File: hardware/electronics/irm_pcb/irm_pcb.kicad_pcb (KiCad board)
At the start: 2 copper layers, 63 parts, among them IC1 23LC1024, J1 Conn_01x04, J10 Conn_02x05_Counter_Clockwise, J11 Conn_01x04, J12 Conn_01x06, J13 Conn_01x06, J14 Conn_01x10, J16 Screw_Terminal_01x02, J17 Conn_01x06, J2 JUMPER_OPEN, J3 JUMPER_CLOSED, J4 JUMPER_CLOSED, J5 AudioJack3_Switch, J6 Screw_Terminal_1x02, J7 Screw_Terminal_1x02, J8 Conn_01x04, J9 Conn_02x15_Top_Bottom, SW1 RST, SW2 0, U1 LM1117-1.8, U2 VS1053B, U3 74LS125, U4 74LS125, U5 ESP32-WROOM-32, U6 LM1117-3.3, U7 TSR1-2450, Y1 12.288MHz

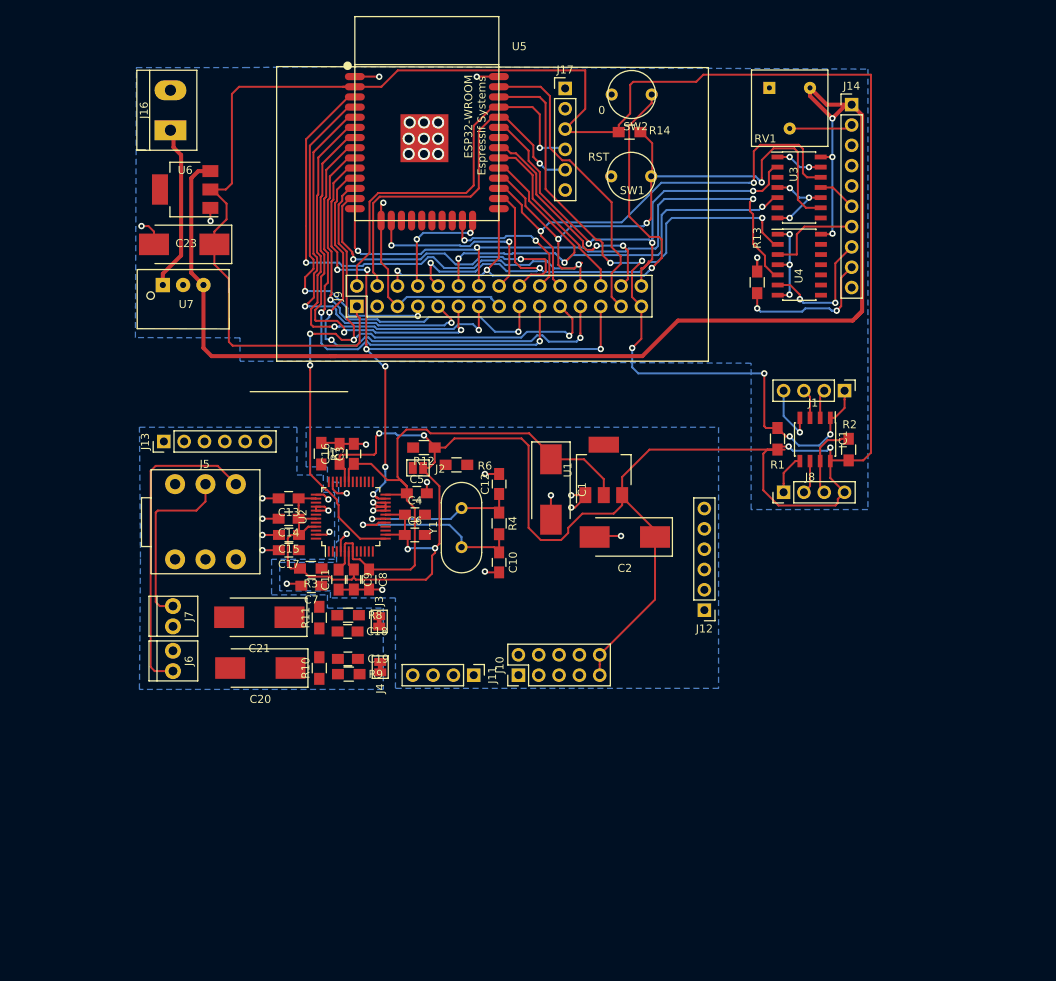
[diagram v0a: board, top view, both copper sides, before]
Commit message: Routing completed
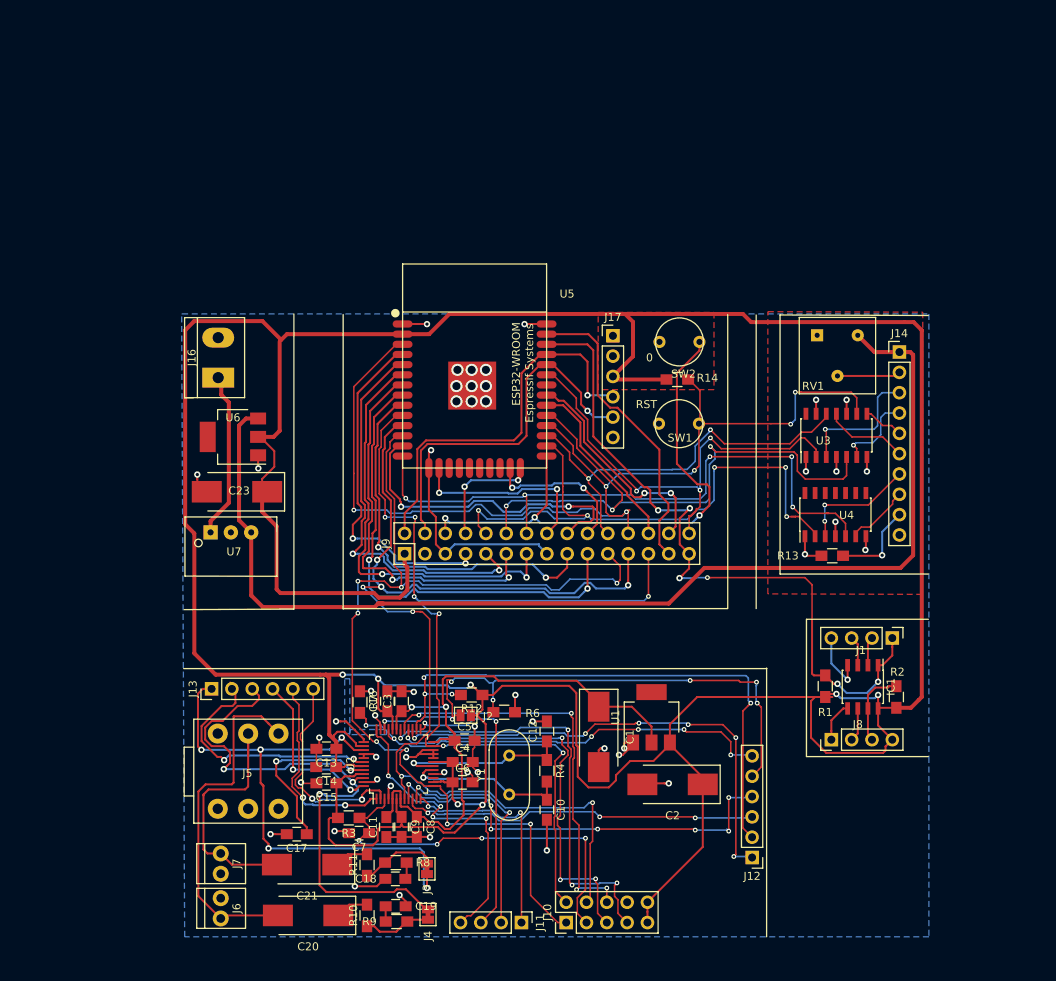
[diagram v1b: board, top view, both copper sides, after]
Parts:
- moved C17 35.5 mm to (101.1, 111.7)
- moved R13 35.4 mm to (168.0, 76.9), turned to 180 degrees
- moved C13 31.7 mm to (104.8, 101.0)
- moved J5 31.6 mm to (95.0, 103.8)
- moved C23 31.6 mm to (93.6, 68.9)
- moved U4 31.6 mm to (168.4, 71.8), turned to 90 degrees
- moved R3 31.5 mm to (107.6, 109.7)
- moved J10 31.5 mm to (134.7, 122.7)
- moved C1 31.5 mm to (138.8, 99.5)
- moved C11 31.5 mm to (112.3, 110.8)
- moved C12 31.5 mm to (132.3, 98.8)
- moved C21 31.5 mm to (102.4, 115.5)
- moved C4 31.5 mm to (121.8, 102.7)
- moved C5 31.5 mm to (122.0, 100.0)
- moved C7 31.5 mm to (108.9, 111.6)
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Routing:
- net +3V3: track 420.3 -> 523.4 mm, vias 6 -> 7
- net /MP3 Codec/DREQ: track 60.5 -> 137.1 mm, vias 3 -> 7
- net /MP3 Codec/RX: track 0.00 -> 73.4 mm, vias 0 -> 4
- net /MP3 Codec/GPIO1: track 0.00 -> 72.0 mm, vias 0 -> 7
- net /MP3 Codec/RIGHT: track 0.00 -> 69.8 mm, vias 0 -> 5
- net /MP3 Codec/LEFT: track 0.00 -> 69.4 mm, vias 0 -> 3
- net /MP3 Codec/TX: track 0.00 -> 60.6 mm, vias 0 -> 6
- net /MP3 Codec/GPIO0: track 0.00 -> 56.3 mm, vias 0 -> 7
- net /MP3 Codec/GPIO2: track 0.00 -> 54.0 mm, vias 0 -> 7
- net /MP3 Codec/SO: track 0.00 -> 54.0 mm, vias 0 -> 4
- net /MP3 Codec/SI: track 0.00 -> 50.5 mm, vias 0 -> 4
- net /MP3 Codec/SCK: track 0.00 -> 50.3 mm, vias 0 -> 4
- net /MP3 Codec/MP3RST: track 0.00 -> 49.0 mm, vias 0 -> 4
- net /MP3 Codec/GPIO3: track 0.00 -> 45.1 mm, vias 0 -> 3
- net /MP3 Codec/LROUT/GPIO4: track 0.00 -> 38.1 mm, vias 0 -> 4
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- added copper zone on F.Cu, net +3V3
- added copper zone on F.Cu, net +5V
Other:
- net class D_Signal added: clearance 0.2, trace_width 0.2, via_dia 0.6, via_drill 0.3

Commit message: Layout completed
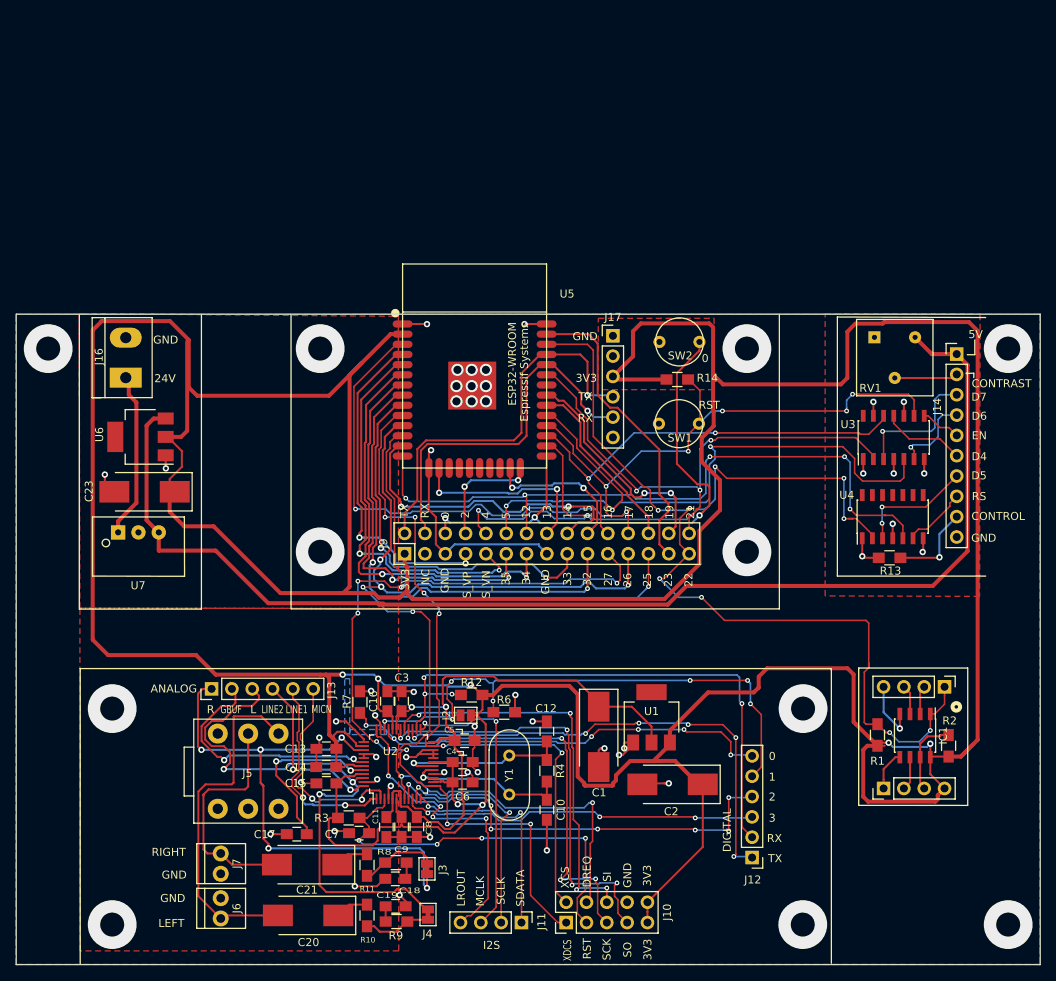
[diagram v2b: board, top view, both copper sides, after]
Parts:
- moved C23 11.6 mm to (82.0, 68.9)
- moved J16 11.6 mm to (79.0, 52.1)
- moved U7 11.6 mm to (78.7, 74.0)
- moved U6 11.6 mm to (81.5, 62.0)
- moved IC1 8.93 mm to (178.4, 99.4)
- moved R2 8.93 mm to (182.5, 100.6)
- moved J8 8.93 mm to (174.4, 106.0)
- moved R1 8.93 mm to (173.7, 99.3)
- moved J1 8.93 mm to (182.0, 93.3)
- moved J14 7.17 mm to (183.6, 51.7)
- moved R13 7.17 mm to (175.2, 77.2)
- moved RV1 7.17 mm to (175.8, 49.6)
- moved U3 7.17 mm to (175.7, 62.1)
- moved U4 7.17 mm to (175.6, 72.0)
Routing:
- net +3V3: track 523.4 -> 671.0 mm
- net /Buffer RAM/RAM-CS: track 88.5 -> 103.3 mm
- net +5V: track 145.0 -> 158.3 mm
- net /Control/D6: track 76.4 -> 83.5 mm
- net /Control/RS: track 79.5 -> 86.6 mm
- net /Control/D5: track 72.7 -> 79.5 mm
- net /Control/D7: track 58.2 -> 64.1 mm
- net /Control/D4: track 51.9 -> 56.6 mm
- net /MP3 Codec/XCS: track 122.4 -> 118.3 mm
- net /Control/EN: track 131.5 -> 135.2 mm, vias 6 -> 7
- net /MP3 Codec/RX: track 73.4 -> 72.0 mm
- net /MP3 Codec/GPIO1: track 72.0 -> 70.7 mm
- net /WROOM Processor/SENSOR_VP: track 43.5 -> 42.4 mm
- net /WROOM Processor/SENSOR_VN: track 49.6 -> 48.6 mm
- net /MP3 Codec/DREQ: track 137.1 -> 136.4 mm
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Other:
- board outline added: 128 x 81.3 mm
- board text added: "1"
- board text added: "12"
- board text added: "13"
- board text added: "14"
- board text added: "15"
- board text added: "16"
- board text added: "17"
- board text added: "18"
- board text added: "19"
- board text added: "2"
- board text added: "21"
- board text added: "22"
- board text added: "23"
- board text added: "24V"
- board text added: "25"
- board text added: "26"
- board text added: "27"
- board text added: "3"
- board text added: "32"
- board text added: "33"
- board text added: "34"
- board text added: "35"
- board text added: "3V3"
- board text added: "4"
- board text added: "5"
- board text added: "5V"
- board text added: "ANALOG"
- board text added: "CONTRAST"
- board text added: "CONTROL"
- board text added: "D4"
- board text added: "D5"
- board text added: "D6"
- board text added: "D7"
- board text added: "DIGITAL"
- board text added: "DREQ"
- board text added: "EN"
- board text added: "GBUF"
- board text added: "GND"
- board text added: "I2S"
- board text added: "L"
- board text added: "LEFT"
- board text added: "LINE1"
- board text added: "LINE2"
- board text added: "LROUT"
- board text added: "MCLK"
- board text added: "MICN"
- board text added: "NC"
- board text added: "R"
- board text added: "RIGHT"
- board text added: "RS"
- board text added: "RX"
- board text added: "SCK"
- board text added: "SCLK"
- board text added: "SDATA"
- board text added: "SI"
- board text added: "SO"
- board text added: "S_VN"
- board text added: "S_VP"
- board text added: "TX"
- board text added: "XCS"
- board text added: "XDCS"
